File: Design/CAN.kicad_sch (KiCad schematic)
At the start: 5 parts

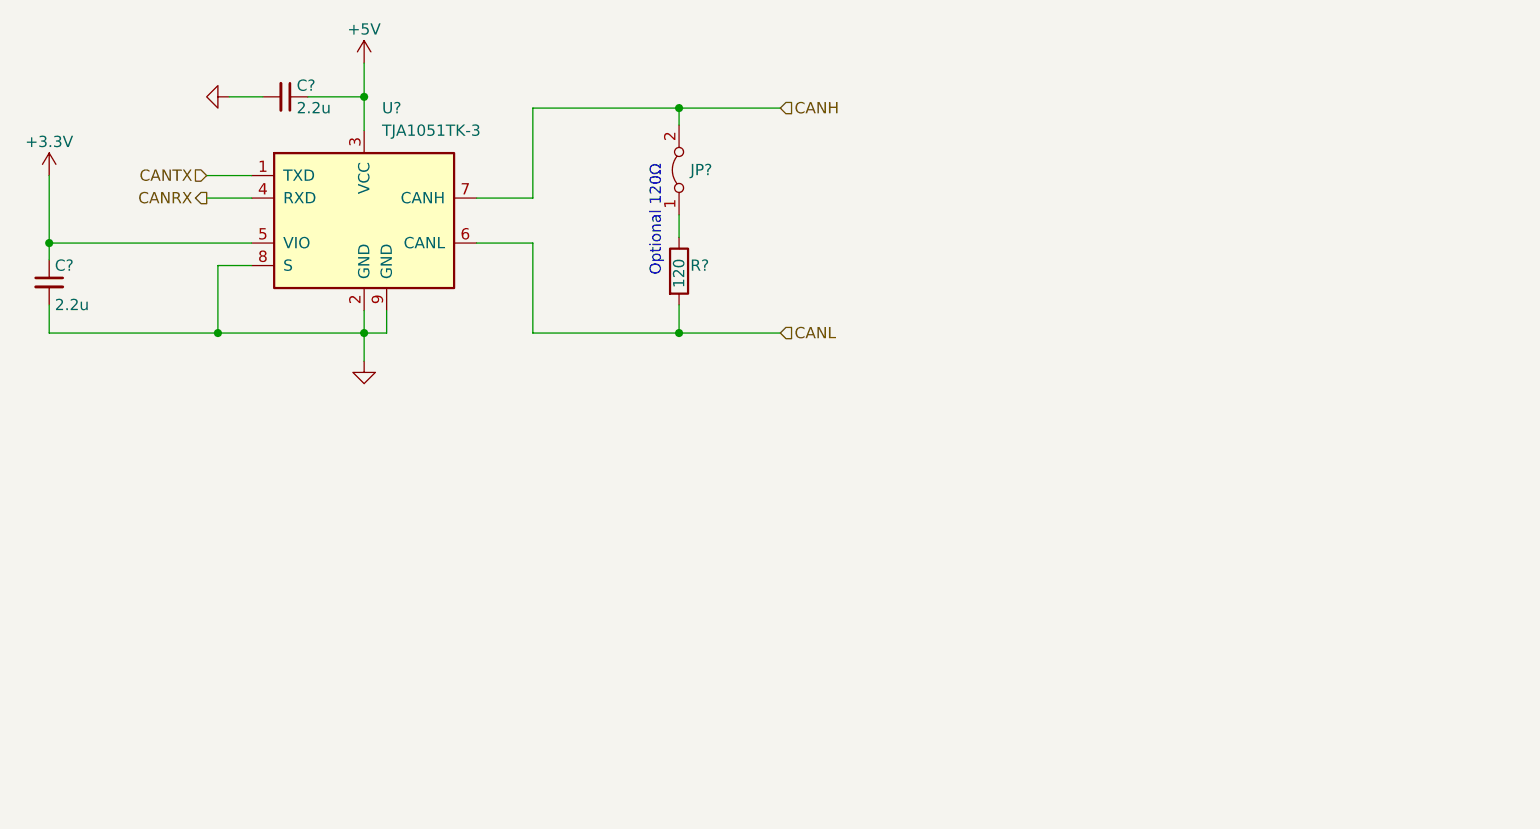
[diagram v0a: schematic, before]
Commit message: schematic updates
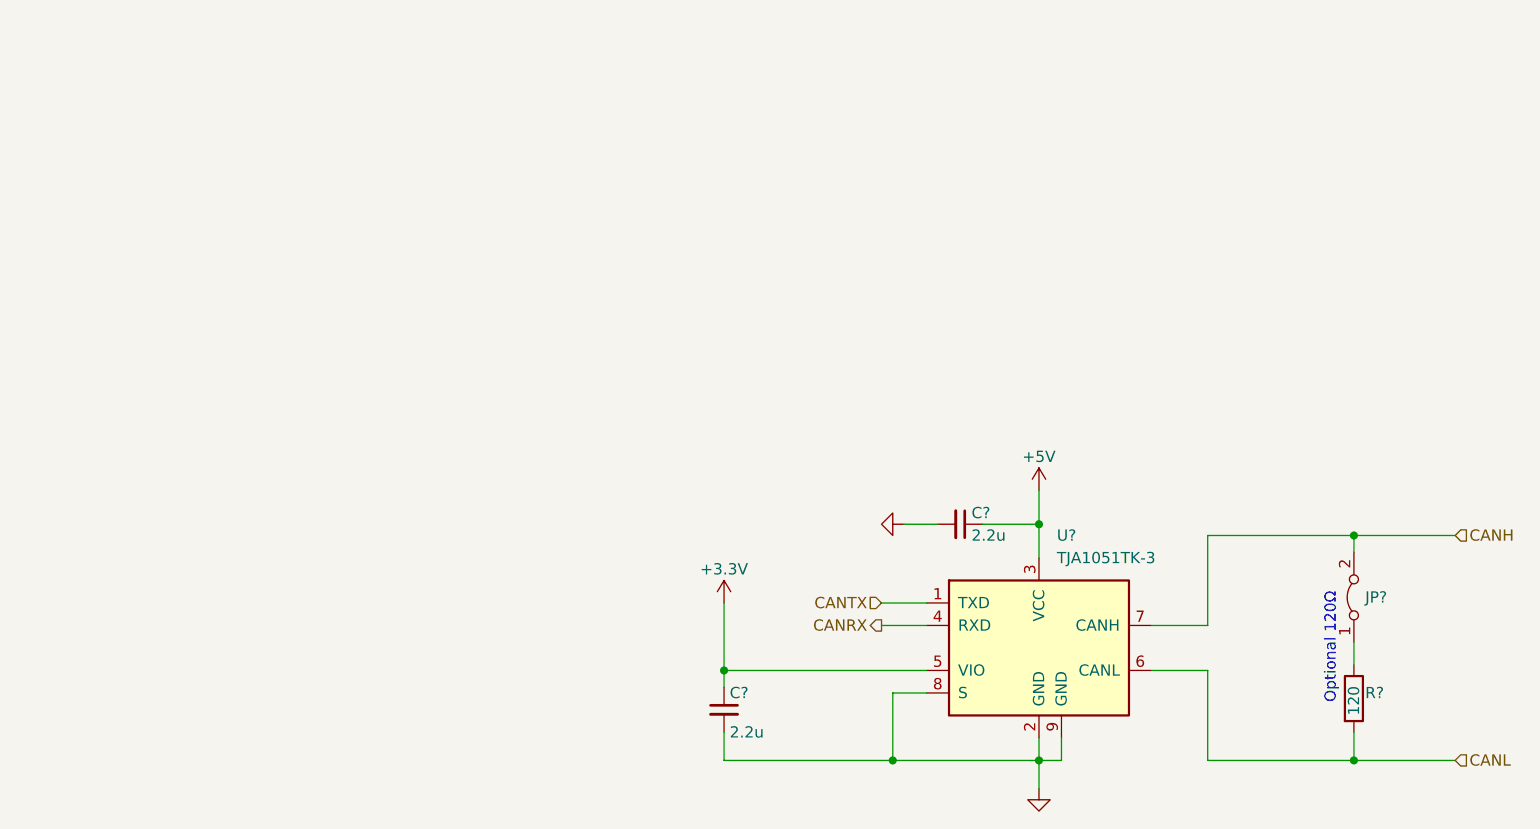
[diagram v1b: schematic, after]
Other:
- moved on the sheet: C?, JP?, R?, U?
